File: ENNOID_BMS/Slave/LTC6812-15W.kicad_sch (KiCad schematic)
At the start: 159 parts, among them J1 PB MB 2, J10 PB MB 1, J11 PA MA 1, J2 PA MA 2, J3 Sensors, J4 Conn_01x08, J5 Conn_01x08, J6 Sensors, Q1 DZTT5551, Q17 DZTT5551, Q18 2N7002, Q19 2N7002, Q20 2N7002, Q21 2N7002, Q22 2N7002, Q23 2N7002, Q24 2N7002, Q25 2N7002, Q26 2N7002, Q27 2N7002, Q28 2N7002, Q29 2N7002, Q30 2N7002, Q31 2N7002, Q32 2N7002, U1 LTC6812-1, U2 LTC6812-1

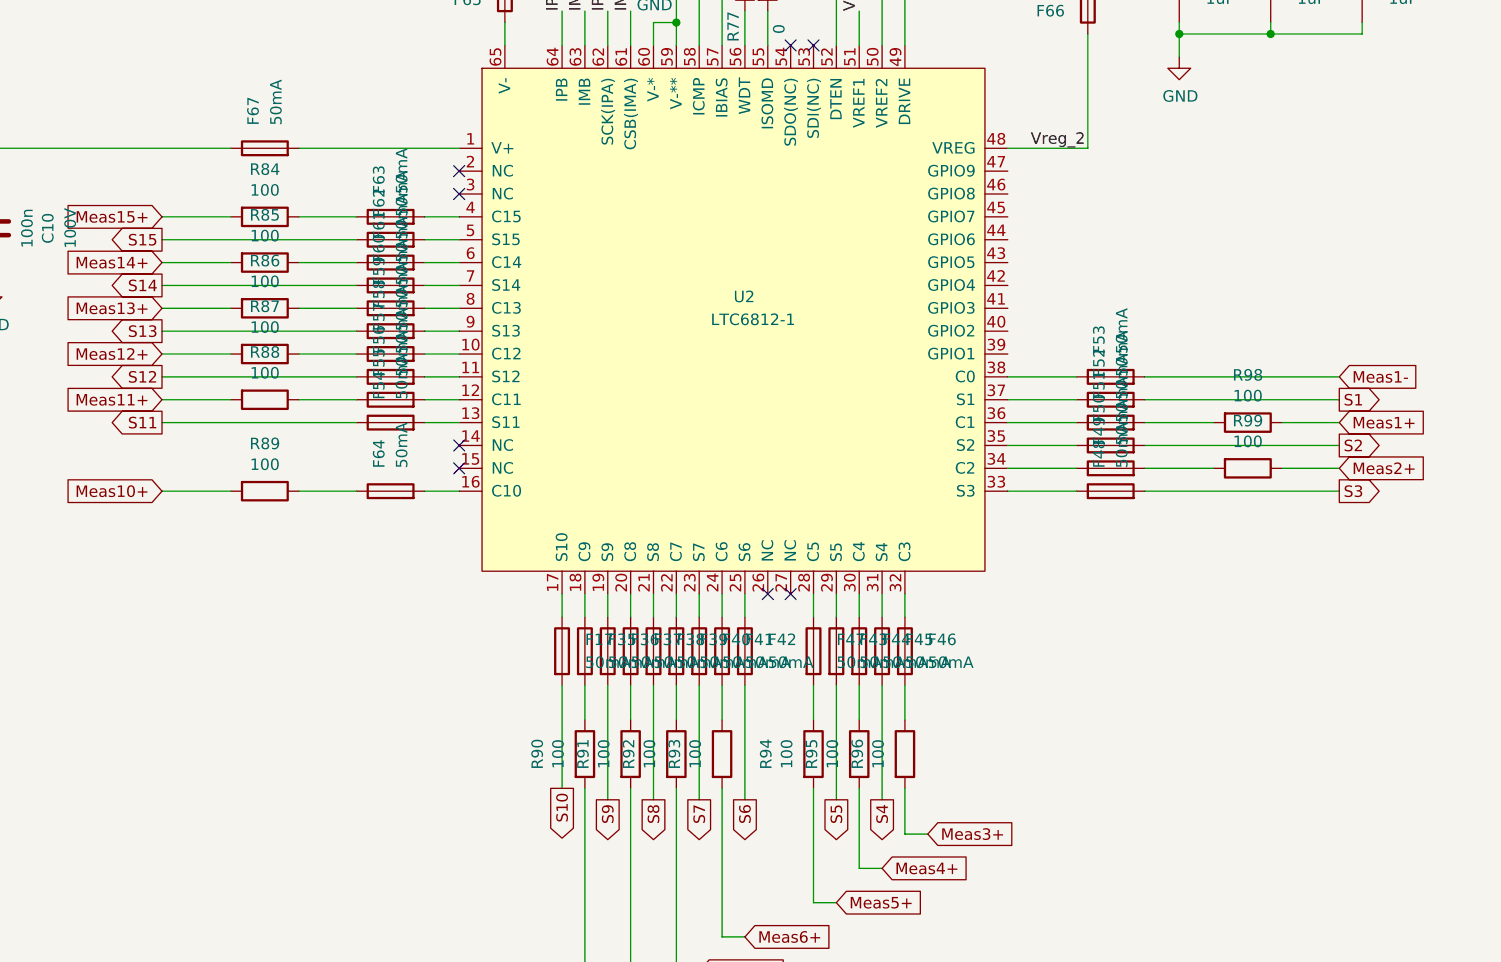
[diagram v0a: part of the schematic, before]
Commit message: fuse boards
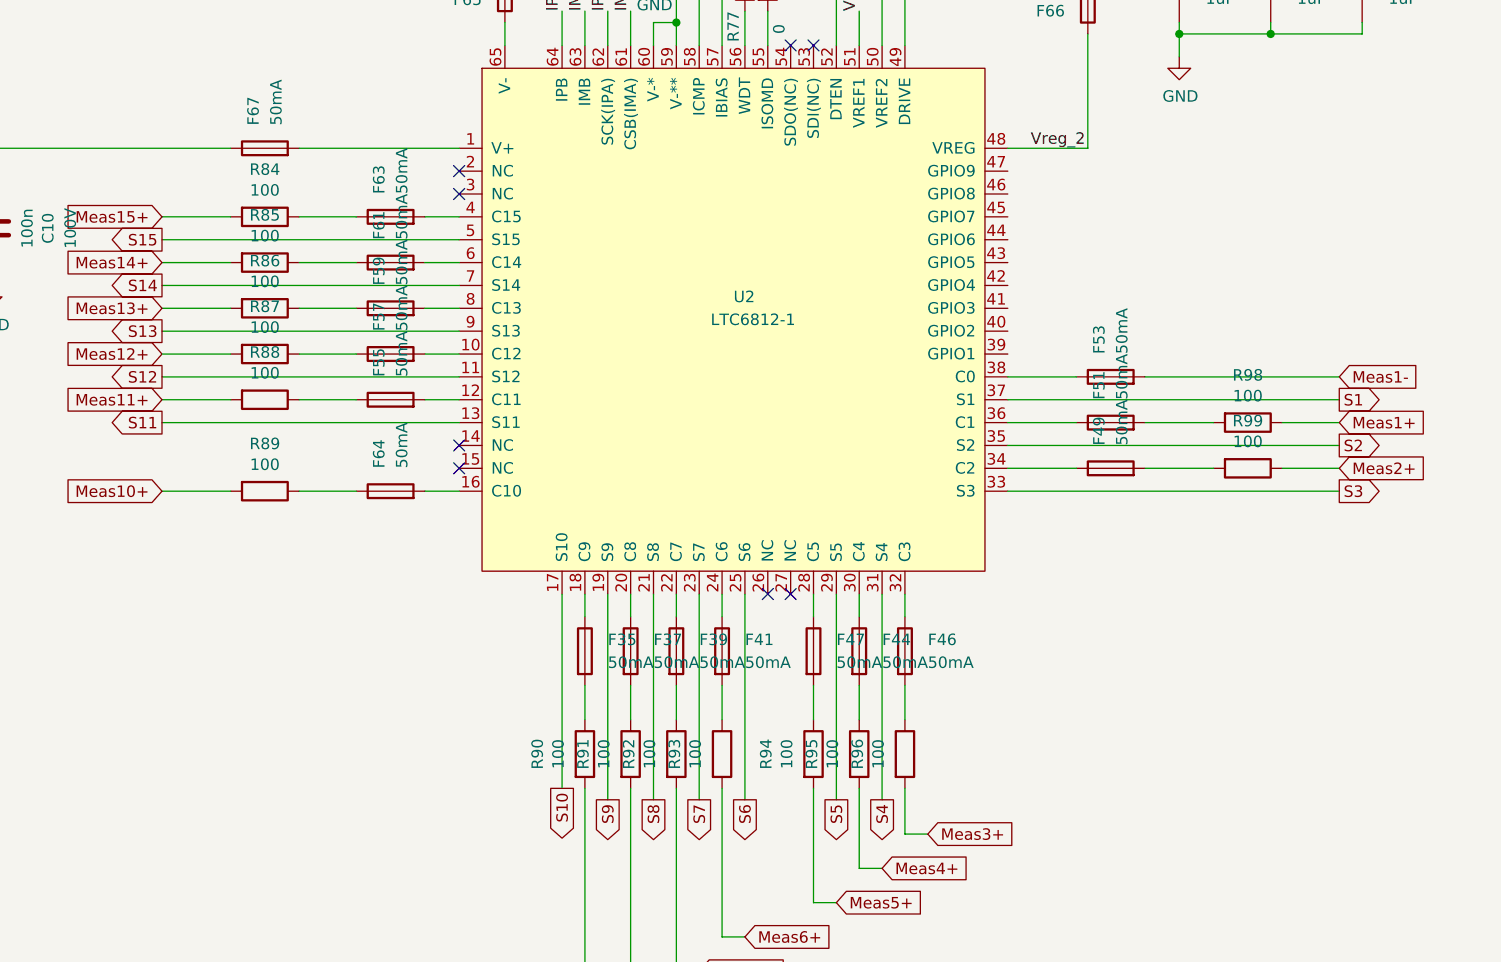
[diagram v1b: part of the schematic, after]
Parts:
- removed F17, F36, F38, F40, F42, F43, F45, F48, F50, F52, F54, F56, F58, F60, F62: 50mA, Fuse:Fuse_0603_1608Metric, symbol Device:Fuse
- R1, R3, R74, R76, R8, R81, R82, R84, R85, R86, R87, R88, R89, R9, R90, R91, R92, R93, R94, R95, R96, R98, R99: Part Number CRCW0603100RFKEA -> RCS0603100RFKEA
- R100, R101, R102, R103, R104, R105, R106, R107, R108, R109, R110, R68, R72, R73, R97: footprint Resistor_SMD:R_0603_1608Metric -> Resistor_SMD:R_0508_1220Metric; Part Number CRCW06033K30FKEA -> WK73R2ATTD3301F
- R11, R12, R16, R20, R24, R28, R32, R36, R40, R44, R48, R52, R56, R60, R64: Part Number ERJ-UP3F6800V -> RCS0603680RFKEA
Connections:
- net S1: now also U2.37 (S1)
- net S10: now also U2.17 (S10)
- net S11: now also U2.13 (S11)
- net S12: now also U2.11 (S12)
- net S13: now also U2.9 (S13)
- net S14: now also U2.7 (S14)
- net S15: now also U2.5 (S15)
- net S2: now also U2.35 (S2)
- net S3: now also U2.33 (S3)
- net S4: now also U2.31 (S4)
- net S5: now also U2.29 (S5)
- net S6: now also U2.25 (S6)
- net S7: now also U2.23 (S7)
- net S8: now also U2.21 (S8)
- net S9: now also U2.19 (S9)
